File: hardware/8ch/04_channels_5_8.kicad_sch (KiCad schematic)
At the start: 0 parts

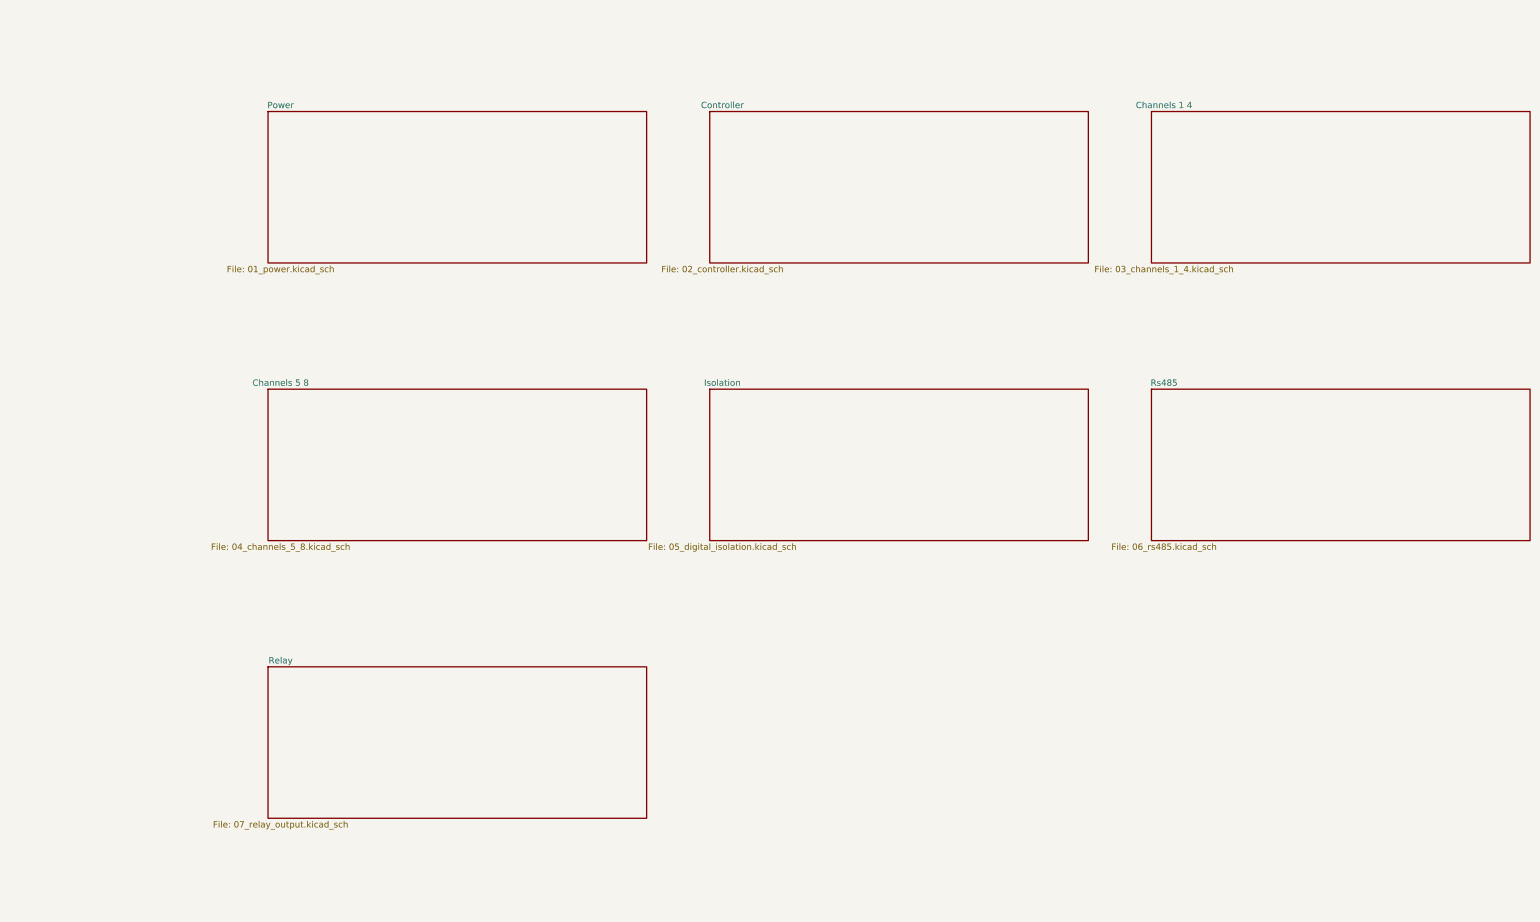
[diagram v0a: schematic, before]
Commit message: fix bugs
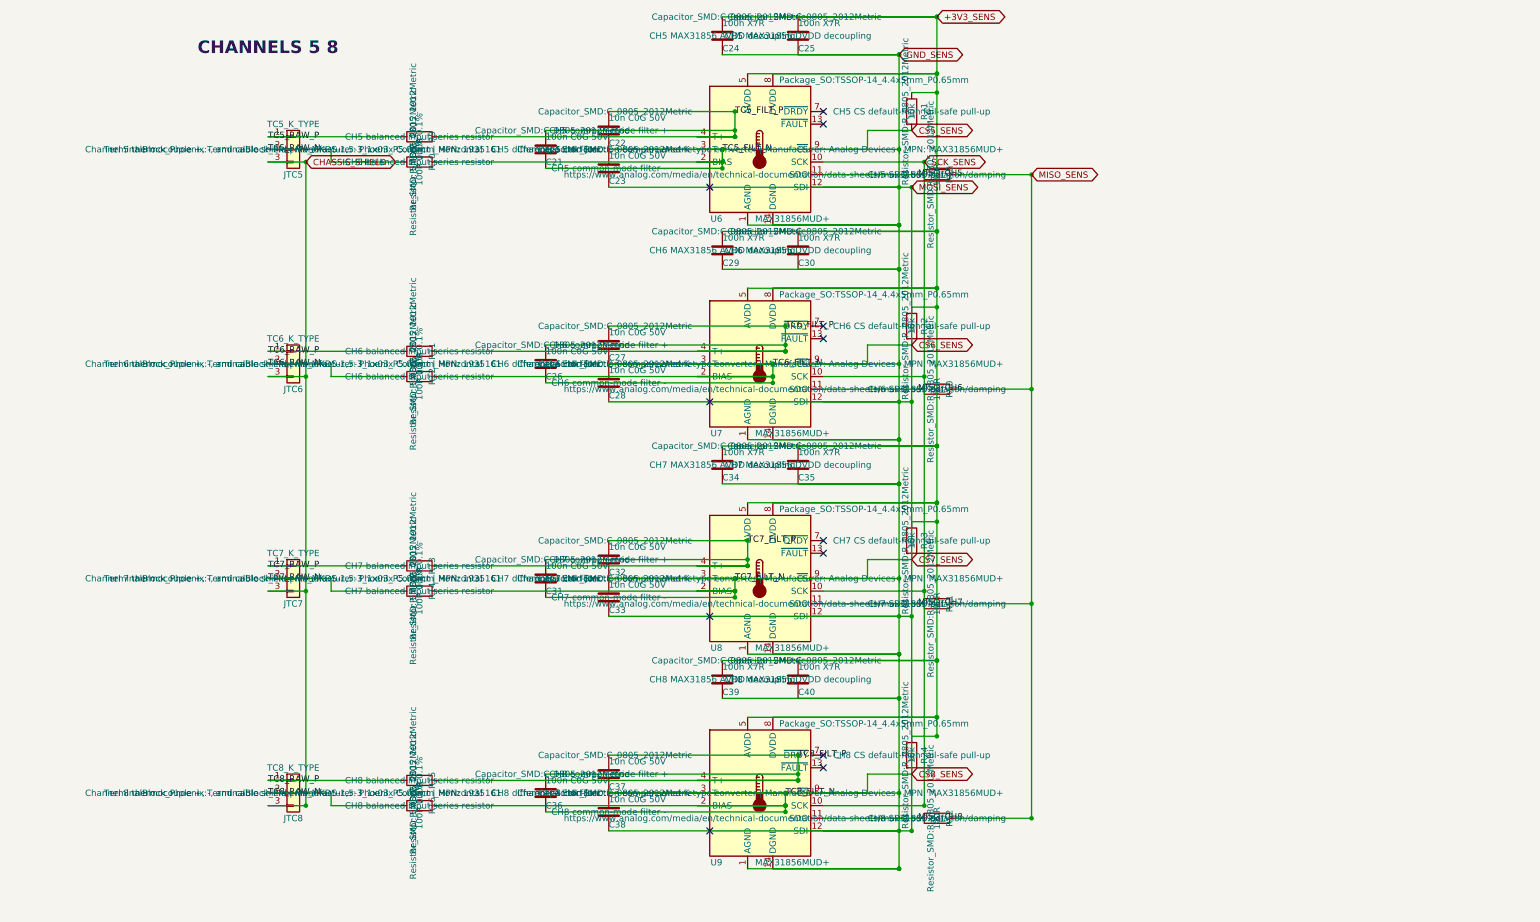
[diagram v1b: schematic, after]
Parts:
- added C21, C26, C31, C36: 100n C0G 50V, Capacitor_SMD:C_0805_2012Metric, symbol Device:C
- added C22, C23, C27, C28, C32, C33, C37, C38: 10n C0G 50V, Capacitor_SMD:C_0805_2012Metric, symbol Device:C
- added C24, C25, C29, C30, C34, C35, C39, C40: 100n X7R, Capacitor_SMD:C_0805_2012Metric, symbol Device:C
- added JTC5: TC5_K_TYPE, TerminalBlock_Phoenix:TerminalBlock_Phoenix_MKDS-1,5-3_1x03_P5.00mm_Horizontal, symbol Connector_Generic:Conn_01x03
- added JTC6: TC6_K_TYPE, TerminalBlock_Phoenix:TerminalBlock_Phoenix_MKDS-1,5-3_1x03_P5.00mm_Horizontal, symbol Connector_Generic:Conn_01x03
- added JTC7: TC7_K_TYPE, TerminalBlock_Phoenix:TerminalBlock_Phoenix_MKDS-1,5-3_1x03_P5.00mm_Horizontal, symbol Connector_Generic:Conn_01x03
- added JTC8: TC8_K_TYPE, TerminalBlock_Phoenix:TerminalBlock_Phoenix_MKDS-1,5-3_1x03_P5.00mm_Horizontal, symbol Connector_Generic:Conn_01x03
- added R10, R11, R12, R13, R14, R15, R16, R9: 100R 0.1%, Resistor_SMD:R_0805_2012Metric, symbol Device:R
- added R21, R22, R23, R24: 10k, Resistor_SMD:R_0805_2012Metric, symbol Device:R
- added R49, R50, R51, R52: 100R, Resistor_SMD:R_0805_2012Metric, symbol Device:R
- added U6, U7, U8, U9: MAX31856MUD+, Package_SO:TSSOP-14_4.4x5mm_P0.65mm, symbol Sensor_Temperature:MAX31856
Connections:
- new net +3V3_SENS: C24.1, C25.1, C29.1, C30.1, C34.1, C35.1, C39.1, C40.1, R21.1, R22.1, R23.1, R24.1, U6.5 (AVDD), U6.8 (DVDD), U7.5 (AVDD), U7.8 (DVDD), U8.5 (AVDD), U8.8 (DVDD), U9.5 (AVDD), U9.8 (DVDD)
- new net CHASSIS_SHIELD: JTC5.3 (Pin_3), JTC6.3 (Pin_3), JTC7.3 (Pin_3), JTC8.3 (Pin_3)
- new net CS5_SENS: C21.2, C22.2, C23.1, C23.2, C24.2, C25.2, C26.2, C27.2, C28.1, C28.2, C29.2, C30.2, C31.2, C32.2, C33.1, C33.2, C34.2, C35.2, C36.2, C37.2, C38.1, C38.2, C39.2, C40.2, R10.2, R12.2, R14.2, R16.2, R21.2, R22.2, R23.2, R24.2, U6.1 (AGND), U6.12 (SDI), U6.14 (DGND), U6.2 (BIAS), U6.3 (T-), U6.9 (~{CS}), U7.1 (AGND), U7.12 (SDI), U7.14 (DGND), U7.2 (BIAS), U7.3 (T-), U7.9 (~{CS}), U8.1 (AGND), U8.12 (SDI), U8.14 (DGND), U8.2 (BIAS), U8.3 (T-), U8.9 (~{CS}), U9.1 (AGND), U9.12 (SDI), U9.14 (DGND), U9.2 (BIAS), U9.3 (T-), U9.9 (~{CS})
- new net MISO_CH5: R49.1, U6.11 (SDO)
- new net MISO_CH6: R50.1, U7.11 (SDO)
- new net MISO_CH7: R51.1, U8.11 (SDO)
- new net MISO_CH8: R52.1, U9.11 (SDO)
- new net MISO_SENS: R49.2, R50.2, R51.2, R52.2
- new net SCK_SENS: U6.10 (SCK), U7.10 (SCK), U8.10 (SCK), U9.10 (SCK)
- new net TC5_FILT_P: C21.1, C22.1, R9.2, U6.4 (T+)
- new net TC5_RAW_N: JTC5.2 (Pin_2), R10.1
- new net TC5_RAW_P: JTC5.1 (Pin_1), R9.1
- new net TC6_FILT_P: C26.1, C27.1, R11.2, U7.4 (T+)
- new net TC6_RAW_N: JTC6.2 (Pin_2), R12.1
- new net TC6_RAW_P: JTC6.1 (Pin_1), R11.1
- new net TC7_FILT_P: C31.1, C32.1, R13.2, U8.4 (T+)
- new net TC7_RAW_N: JTC7.2 (Pin_2), R14.1
- new net TC7_RAW_P: JTC7.1 (Pin_1), R13.1
- new net TC8_FILT_P: C36.1, C37.1, R15.2, U9.4 (T+)
- new net TC8_RAW_N: JTC8.2 (Pin_2), R16.1
- new net TC8_RAW_P: JTC8.1 (Pin_1), R15.1
- no-connect marks 0 -> 12
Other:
- removed sheet Channels 1 4
- removed sheet Channels 5 8
- removed sheet Controller
- removed sheet Isolation
- removed sheet Power
- removed sheet Relay
- removed sheet Rs485
- note added: "CHANNELS 5 8"
